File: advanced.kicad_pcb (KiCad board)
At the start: 2 copper layers, 99.8 x 99.8 mm, 108 parts, among them U1 ATtiny24-20P, U2 ATtiny28L-4P, U3 ATtiny13A-P, U4 ATtiny25-20P, U5 ATtiny24-20P, U6 ATtiny85-20P

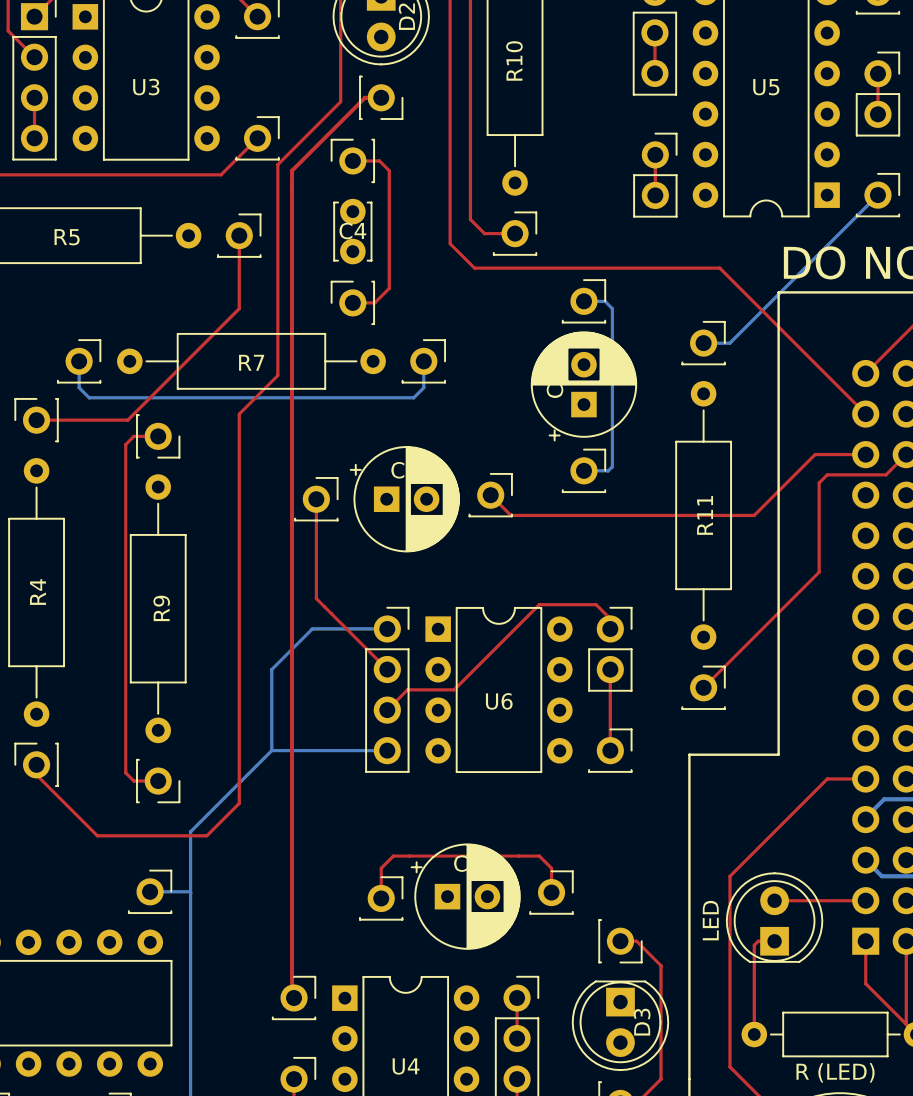
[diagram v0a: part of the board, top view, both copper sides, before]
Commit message: DGRS
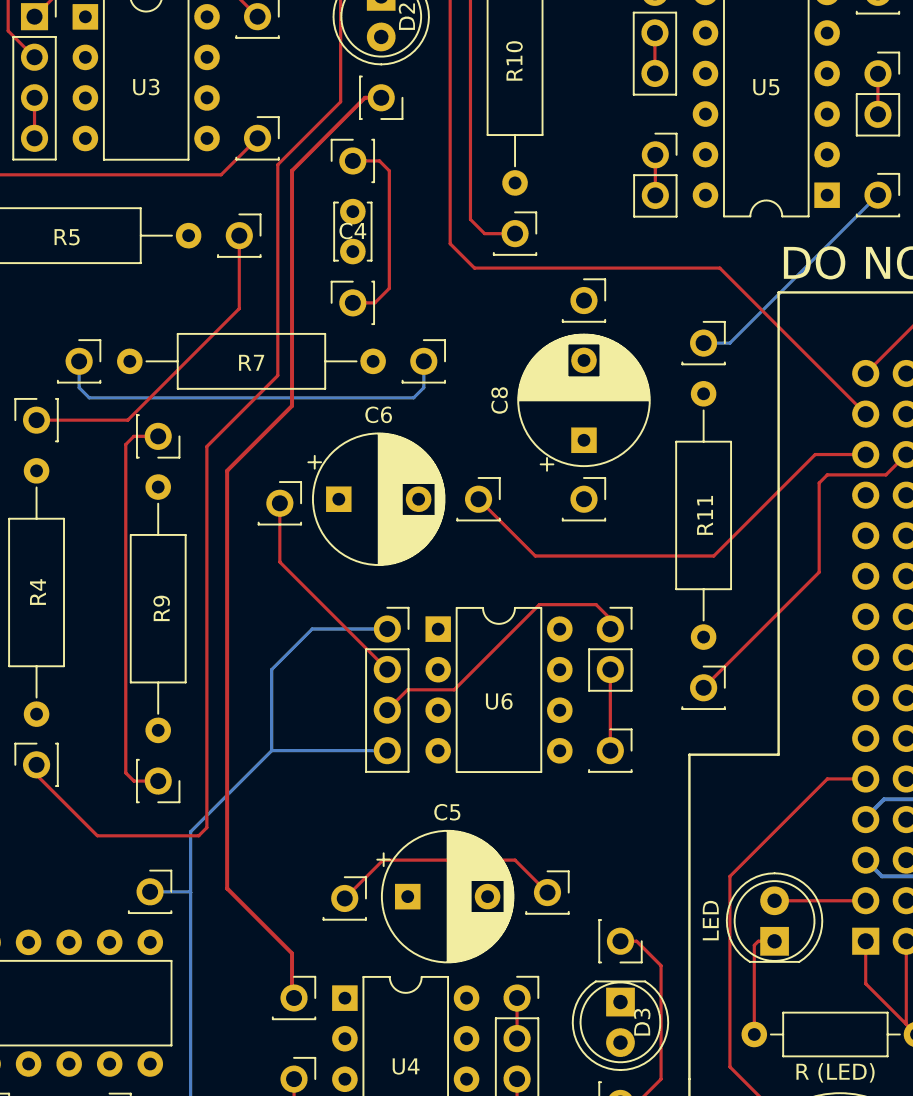
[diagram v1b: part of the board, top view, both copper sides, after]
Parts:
- C5, C6, C8: footprint Capacitor_THT:CP_Radial_D6.3mm_P2.50mm -> Capacitor_THT:CP_Radial_D8.0mm_P5.00mm
- moved C6 3.00 mm to (212.7, 101.9)
- moved C5 2.49 mm to (217.1, 126.7)
- moved   2.30 mm to (209.0, 102.1)
- moved   2.29 mm to (213.1, 126.9)
- moved C8 2.24 mm to (228.1, 98.2)
- moved   1.78 mm to (228.1, 101.9)
- moved   0.80 mm to (221.5, 101.9)
- moved   0.25 mm to (225.8, 126.5)
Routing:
- net (no net): track 1721.8 -> 1714.4 mm
